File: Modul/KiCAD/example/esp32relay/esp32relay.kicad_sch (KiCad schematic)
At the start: 18 parts, among them J1 Conn_01x03_Male, J2 Conn_01x02_Male, SW1 SW_Push, SW2 SW_Push, U1 ESP32-WROOM-32, U2 AMS1117-3.3

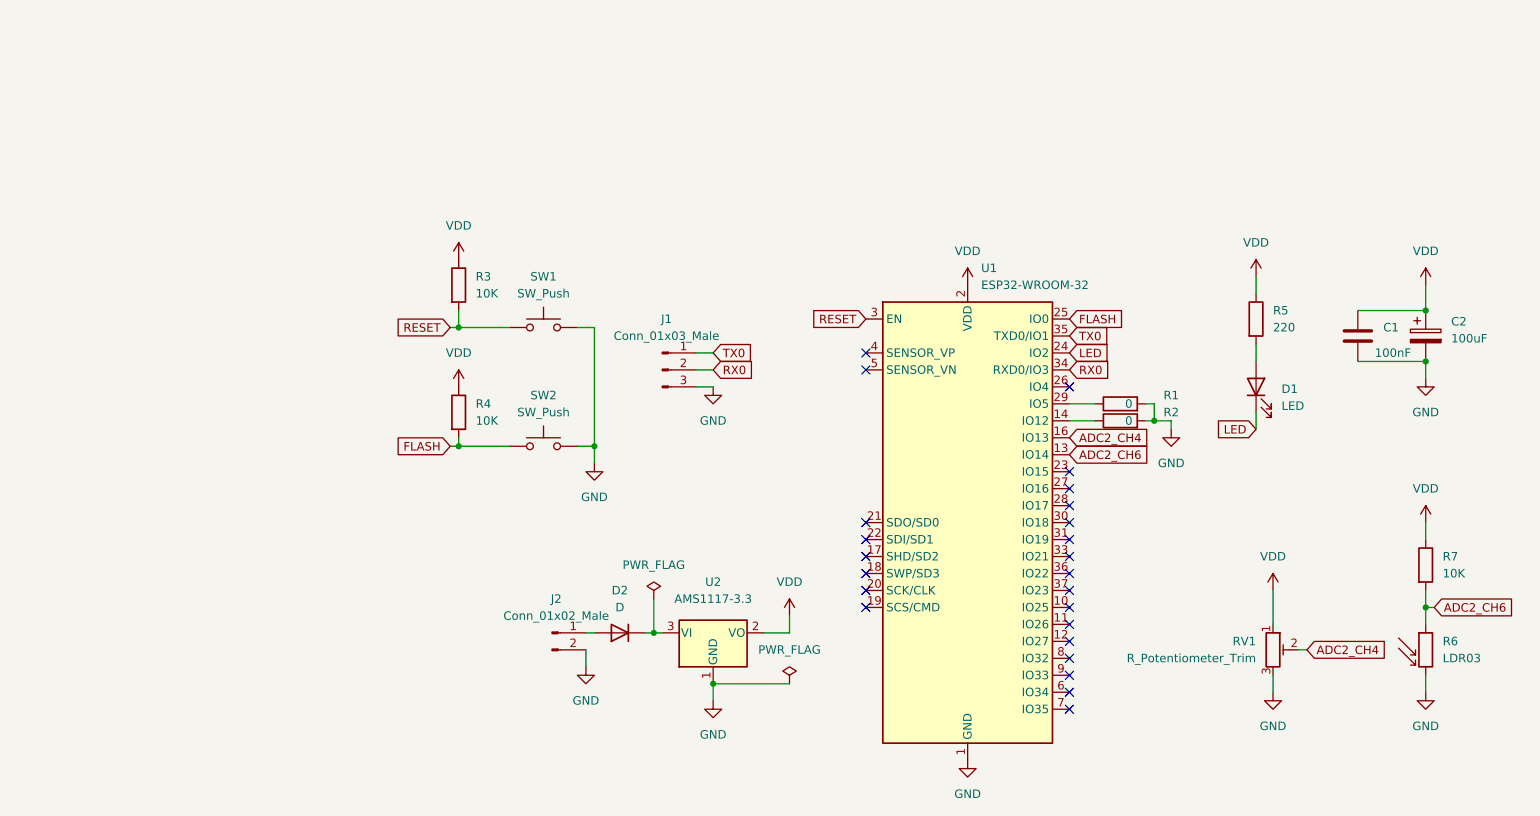
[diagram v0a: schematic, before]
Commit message: KiCAD Sch
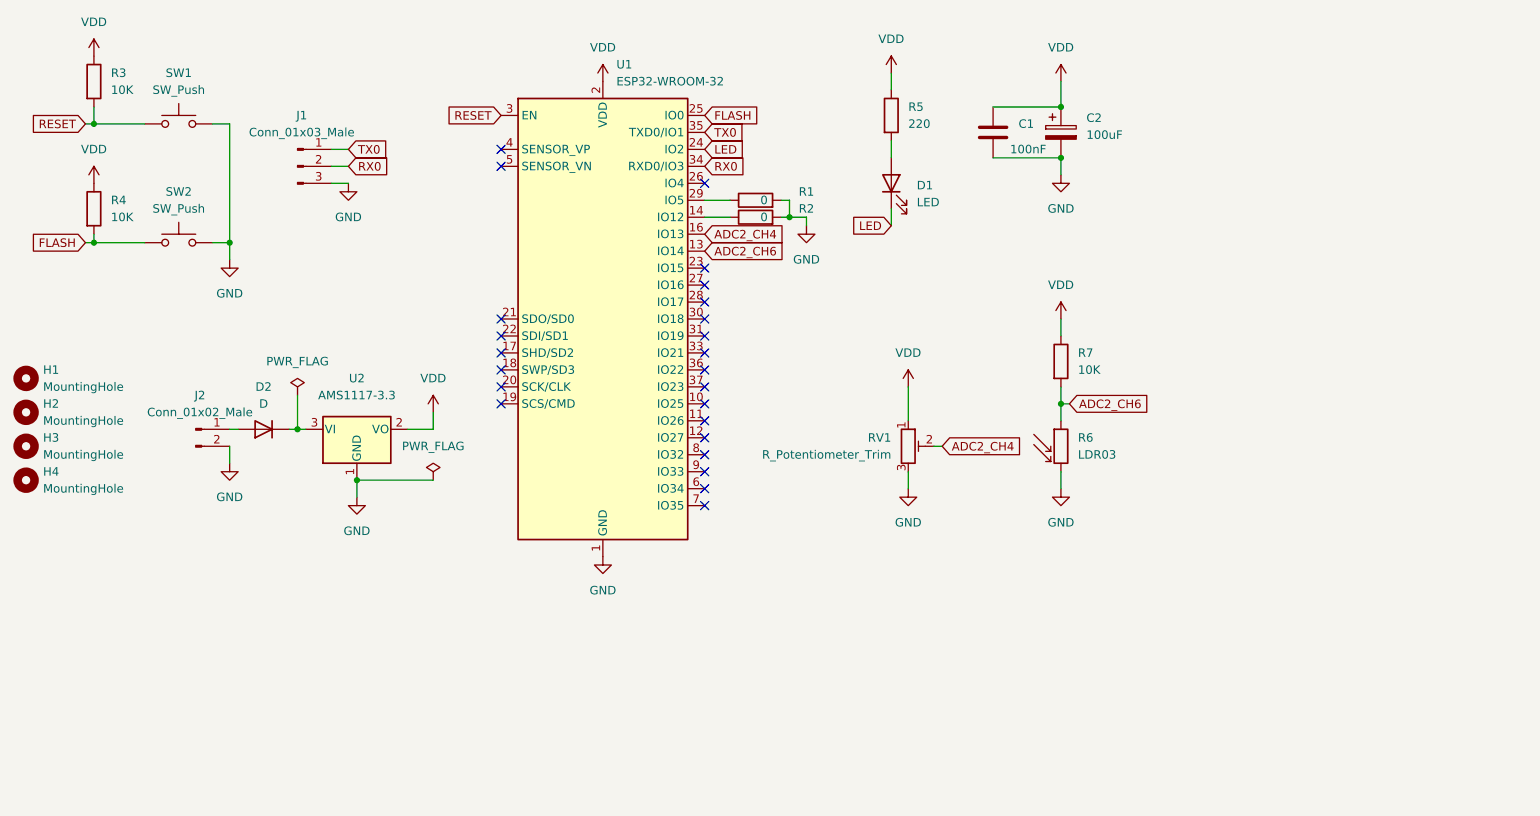
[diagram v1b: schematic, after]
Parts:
- added H1, H2, H3, H4: MountingHole, symbol Mechanical:MountingHole
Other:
- company: (none) -> PT Mencari Cinta Sejati by Achmadi ST MT
- title: (none) -> KiCAD Example 
- moved on the sheet: C1, C2, D1, D2, J1, J2, R1, R2, R3, R4, R5, R6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

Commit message: KiCAD Footprint Assigment
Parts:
- C1, C2: footprint (none) -> Capacitor_SMD:C_0805_2012Metric
- D1: footprint (none) -> LED_SMD:LED_0805_2012Metric
- D2: footprint (none) -> Diode_SMD:D_SMA
- H1, H2, H3, H4: footprint (none) -> MountingHole:MountingHole_2.5mm_Pad_Via
- J1: footprint (none) -> Connector_PinHeader_2.54mm:PinHeader_1x03_P2.54mm_Horizontal
- J2: footprint (none) -> TerminalBlock_Altech:Altech_AK300_1x02_P5.00mm_45-Degree
- R1, R2, R3, R4, R5, R7: footprint (none) -> Resistor_SMD:R_0805_2012Metric
- RV1: footprint (none) -> Potentiometer_SMD:Potentiometer_Vishay_TS53YJ_Vertical
- SW1, SW2: footprint (none) -> Button_Switch_THT:SW_PUSH_6mm
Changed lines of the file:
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@@
       (effects (font (size 1.27 1.27)) (justify right))
     )
-    (property "Footprint" "" (id 2) (at 146.05 40.64 0)
+    (property "Footprint" "LED_SMD:LED_0805_2012Metric" (id 2) (at 146.05 40.64 0)
       (effects (font (size 1.27 1.27)) hide)
     )
@@
       (effects (font (size 1.27 1.27)) (justify left))
     )
-    (property "Footprint" "" (id 2) (at 16.51 85.09 0)
+    (property "Footprint" "MountingHole:MountingHole_2.5mm_Pad_Via" (id 2) (at 16.51 85.09 0)
       (effects (font (size 1.27 1.27)) hide)
     )
@@
       (effects (font (size 1.27 1.27)) (justify right))
     )
-    (property "Footprint" "" (id 2) (at 148.59 80.01 0)
+    (property "Footprint" "Potentiometer_SMD:Potentiometer_Vishay_TS53YJ_Vertical" (id 2) (at 148.59 80.01 0)
       (effects (font (size 1.27 1.27)) hide)
     )
@@
       (effects (font (size 1.27 1.27)) (justify left))
     )
-    (property "Footprint" "" (id 2) (at 144.272 30.48 90)
+    (property "Footprint" "Resistor_SMD:R_0805_2012Metric" (id 2) (at 144.272 30.48 90)
       (effects (font (size 1.27 1.27)) hide)
     )
@@
       (effects (font (size 1.27 1.27)) (justify left))
     )
-    (property "Footprint" "" (id 2) (at 16.51 74.93 0)
+    (property "Footprint" "MountingHole:MountingHole_2.5mm_Pad_Via" (id 2) (at 16.51 74.93 0)
       (effects (font (size 1.27 1.27)) hide)
     )
@@
       (effects (font (size 1.27 1.27)) (justify left))
     )
-    (property "Footprint" "" (id 2) (at 162.2552 36.83 0)
+    (property "Footprint" "Capacitor_SMD:C_0805_2012Metric" (id 2) (at 162.2552 36.83 0)
       (effects (font (size 1.27 1.27)) hide)
     )
@@
       (effects (font (size 1.27 1.27)) (justify left))
     )
-    (property "Footprint" "" (id 2) (at 24.892 44.45 90)
+    (property "Footprint" "Resistor_SMD:R_0805_2012Metric" (id 2) (at 24.892 44.45 90)
       (effects (font (size 1.27 1.27)) hide)
     )
@@
       (effects (font (size 1.27 1.27)) (justify left))
     )
-    (property "Footprint" "" (id 2) (at 169.672 67.31 90)
+    (property "Footprint" "Resistor_SMD:R_0805_2012Metric" (id 2) (at 169.672 67.31 90)
       (effects (font (size 1.27 1.27)) hide)
     )
@@
     (property "Reference" "J2" (id 0) (at 42.545 72.39 0))
     (property "Value" "Conn_01x02_Male" (id 1) (at 42.545 74.93 0))
-    (property "Footprint" "" (id 2) (at 41.91 77.47 0)
+    (property "Footprint" "TerminalBlock_Altech:Altech_AK300_1x02_P5.00mm_45-Degree" (id 2) (at 41.91 77.47 0)
       (effects (font (size 1.27 1.27)) hide)
     )
@@
     (property "Reference" "D2" (id 0) (at 52.07 71.12 0))
     (property "Value" "D" (id 1) (at 52.07 73.66 0))
-    (property "Footprint" "" (id 2) (at 52.07 77.47 0)
+    (property "Footprint" "Diode_SMD:D_SMA" (id 2) (at 52.07 77.47 0)
       (effects (font (size 1.27 1.27)) hide)
     )
@@
     (property "Reference" "J1" (id 0) (at 57.785 30.48 0))
     (property "Value" "Conn_01x03_Male" (id 1) (at 57.785 33.02 0))
-    (property "Footprint" "" (id 2) (at 57.15 38.1 0)
+    (property "Footprint" "Connector_PinHeader_2.54mm:PinHeader_1x03_P2.54mm_Horizontal" (id 2) (at 57.15 38.1 0)
       (effects (font (size 1.27 1.27)) hide)
     )
@@
       (effects (font (size 1.27 1.27)) (justify left))
     )
-    (property "Footprint" "" (id 2) (at 16.51 69.85 0)
+    (property "Footprint" "MountingHole:MountingHole_2.5mm_Pad_Via" (id 2) (at 16.51 69.85 0)
       (effects (font (size 1.27 1.27)) hide)
     )
@@
       (effects (font (size 1.27 1.27)) (justify left))
     )
-    (property "Footprint" "" (id 2) (at 172.4152 36.83 0)
+    (property "Footprint" "Capacitor_SMD:C_0805_2012Metric" (id 2) (at 172.4152 36.83 0)
       (effects (font (size 1.27 1.27)) hide)
     )
@@
       (effects (font (size 1.27 1.27)) (justify left))
     )
-    (property "Footprint" "" (id 2) (at 24.892 25.4 90)
+    (property "Footprint" "Resistor_SMD:R_0805_2012Metric" (id 2) (at 24.892 25.4 90)
       (effects (font (size 1.27 1.27)) hide)
     )
@@
     (property "Reference" "R2" (id 0) (at 133.35 44.45 90))
     (property "Value" "0" (id 1) (at 127 45.72 90))
-    (property "Footprint" "" (id 2) (at 125.73 47.498 90)
+    (property "Footprint" "Resistor_SMD:R_0805_2012Metric" (id 2) (at 125.73 47.498 90)
       (effects (font (size 1.27 1.27)) hide)
     )
@@
     (property "Reference" "R1" (id 0) (at 133.35 41.91 90))
     (property "Value" "0" (id 1) (at 127 43.18 90))
-    (property "Footprint" "" (id 2) (at 125.73 44.958 90)
+    (property "Footprint" "Resistor_SMD:R_0805_2012Metric" (id 2) (at 125.73 44.958 90)
       (effects (font (size 1.27 1.27)) hide)
     )
@@
     (property "Reference" "SW2" (id 0) (at 39.37 41.91 0))
     (property "Value" "SW_Push" (id 1) (at 39.37 44.45 0))
-    (property "Footprint" "" (id 2) (at 39.37 44.45 0)
+    (property "Footprint" "Button_Switch_THT:SW_PUSH_6mm" (id 2) (at 39.37 44.45 0)
       (effects (font (size 1.27 1.27)) hide)
     )
@@
     (property "Reference" "SW1" (id 0) (at 39.37 24.13 0))
     (property "Value" "SW_Push" (id 1) (at 39.37 26.67 0))
-    (property "Footprint" "" (id 2) (at 39.37 26.67 0)
+    (property "Footprint" "Button_Switch_THT:SW_PUSH_6mm" (id 2) (at 39.37 26.67 0)
       (effects (font (size 1.27 1.27)) hide)
     )
@@
       (effects (font (size 1.27 1.27)) (justify left))
     )
-    (property "Footprint" "" (id 2) (at 16.51 80.01 0)
+    (property "Footprint" "MountingHole:MountingHole_2.5mm_Pad_Via" (id 2) (at 16.51 80.01 0)
       (effects (font (size 1.27 1.27)) hide)
     )
@@
     )
     (path "/4a03fd8d-7351-40da-89c3-276811b60f6c"
-      (reference "C1") (unit 1) (value "100nF") (footprint "")
+      (reference "C1") (unit 1) (value "100nF") (footprint "Capacitor_SMD:C_0805_2012Metric")
     )
     (path "/c9a3ea59-03f3-4e5f-b974-94bba4eeb410"
-      (reference "C2") (unit 1) (value "100uF") (footprint "")
+      (reference "C2") (unit 1) (value "100uF") (footprint "Capacitor_SMD:C_0805_2012Metric")
     )
     (path "/08ca79ae-1d3d-49da-9188-4200a6d96315"
-      (reference "D1") (unit 1) (value "LED") (footprint "")
+      (reference "D1") (unit 1) (value "LED") (footprint "LED_SMD:LED_0805_2012Metric")
     )
     (path "/86c3c232-c513-44d1-b2c2-ad6d48cdc8bd"
-      (reference "D2") (unit 1) (value "D") (footprint "")
+      (reference "D2") (unit 1) (value "D") (footprint "Diode_SMD:D_SMA")
     )
     (path "/bb32ba3d-3e21-4f3f-8204-e499aec217cb"
-      (reference "H1") (unit 1) (value "MountingHole") (footprint "")
+      (reference "H1") (unit 1) (value "MountingHole") (footprint "MountingHole:MountingHole_2.5mm_Pad_Via")
     )
     (path "/3bc9da20-1b84-498d-a371-dd139a1a349b"
-      (reference "H2") (unit 1) (value "MountingHole") (footprint "")
+      (reference "H2") (unit 1) (value "MountingHole") (footprint "MountingHole:MountingHole_2.5mm_Pad_Via")
     )
     (path "/f9b2aae8-f7c5-4890-8208-9244c6d31b97"
-      (reference "H3") (unit 1) (value "MountingHole") (footprint "")
+      (reference "H3") (unit 1) (value "MountingHole") (footprint "MountingHole:MountingHole_2.5mm_Pad_Via")
     )
     (path "/0950750a-20b6-41a2-b0de-a92dd2be1301"
-      (reference "H4") (unit 1) (value "MountingHole") (footprint "")
+      (reference "H4") (unit 1) (value "MountingHole") (footprint "MountingHole:MountingHole_2.5mm_Pad_Via")
     )
     (path "/b001b016-75d8-4e79-9b6f-c741feb2c038"
-      (reference "J1") (unit 1) (value "Conn_01x03_Male") (footprint "")
+      (reference "J1") (unit 1) (value "Conn_01x03_Male") (footprint "Connector_PinHeader_2.54mm:PinHeader_1x03_P2.54mm_Horizontal")
     )
     (path "/63068f0a-7295-4fd8-8d22-9f943575f98f"
-      (reference "J2") (unit 1) (value "Conn_01x02_Male") (footprint "")
+      (reference "J2") (unit 1) (value "Conn_01x02_Male") (footprint "TerminalBlock_Altech:Altech_AK300_1x02_P5.00mm_45-Degree")
     )
     (path "/dbf46492-5832-4a0d-bd29-77f6c79624b3"
-      (reference "R1") (unit 1) (value "0") (footprint "")
+      (reference "R1") (unit 1) (value "0") (footprint "Resistor_SMD:R_0805_2012Metric")
     )
     (path "/d91585d4-7c1e-422b-9a0c-f2f496c95b30"
-      (reference "R2") (unit 1) (value "0") (footprint "")
+      (reference "R2") (unit 1) (value "0") (footprint "Resistor_SMD:R_0805_2012Metric")
     )
     (path "/ca46a2e3-c402-4de8-953d-f424598095e7"
-      (reference "R3") (unit 1) (value "10K") (footprint "")
+      (reference "R3") (unit 1) (value "10K") (footprint "Resistor_SMD:R_0805_2012Metric")
     )
     (path "/4ff203d8-d747-4e5e-b3f9-172370dc9d4b"
-      (reference "R4") (unit 1) (value "10K") (footprint "")
+      (reference "R4") (unit 1) (value "10K") (footprint "Resistor_SMD:R_0805_2012Metric")
     )
     (path "/3937687f-ec32-4a2a-8367-a3d0aa3800b0"
-      (reference "R5") (unit 1) (value "220") (footprint "")
+      (reference "R5") (unit 1) (value "220") (footprint "Resistor_SMD:R_0805_2012Metric")
     )
     (path "/d2e80b94-3249-40ce-8c31-151dfee98587"
@@
     )
     (path "/588512c4-4c95-4ce2-a4f2-d94022531a13"
-      (reference "R7") (unit 1) (value "10K") (footprint "")
+      (reference "R7") (unit 1) (value "10K") (footprint "Resistor_SMD:R_0805_2012Metric")
     )
     (path "/270ec5b1-ad3d-48dc-953f-492a211115e8"
-      (reference "RV1") (unit 1) (value "R_Potentiometer_Trim") (footprint "")
+      (reference "RV1") (unit 1) (value "R_Potentiometer_Trim") (footprint "Potentiometer_SMD:Potentiometer_Vishay_TS53YJ_Vertical")
     )
     (path "/f7f5136e-6a60-41f6-a84f-3fa52bfc06fb"
-      (reference "SW1") (unit 1) (value "SW_Push") (footprint "")
+      (reference "SW1") (unit 1) (value "SW_Push") (footprint "Button_Switch_THT:SW_PUSH_6mm")
     )
     (path "/f4430897-22d3-4c1d-98b5-2d7ed72eb632"
-      (reference "SW2") (unit 1) (value "SW_Push") (footprint "")
+      (reference "SW2") (unit 1) (value "SW_Push") (footprint "Button_Switch_THT:SW_PUSH_6mm")
     )
     (path "/4376e9d3-2a99-4b53-a419-76ef318ac824"
